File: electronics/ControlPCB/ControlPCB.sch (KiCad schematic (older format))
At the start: 29 parts, among them CON1 BARREL_JACK, P1 Opto1, P2 Opto2, P3 Opto3, P4 Opto4, P5 Opto5, P6 Opto6, P7 Tool, U1 POLOLU_A4988, U2 POLOLU_A4988, U3 POLOLU_A4988, U4 POLOLU_A4988, U5 POLOLU_A4988, U6 POLOLU_A4988, U7 POLOLU_A4988

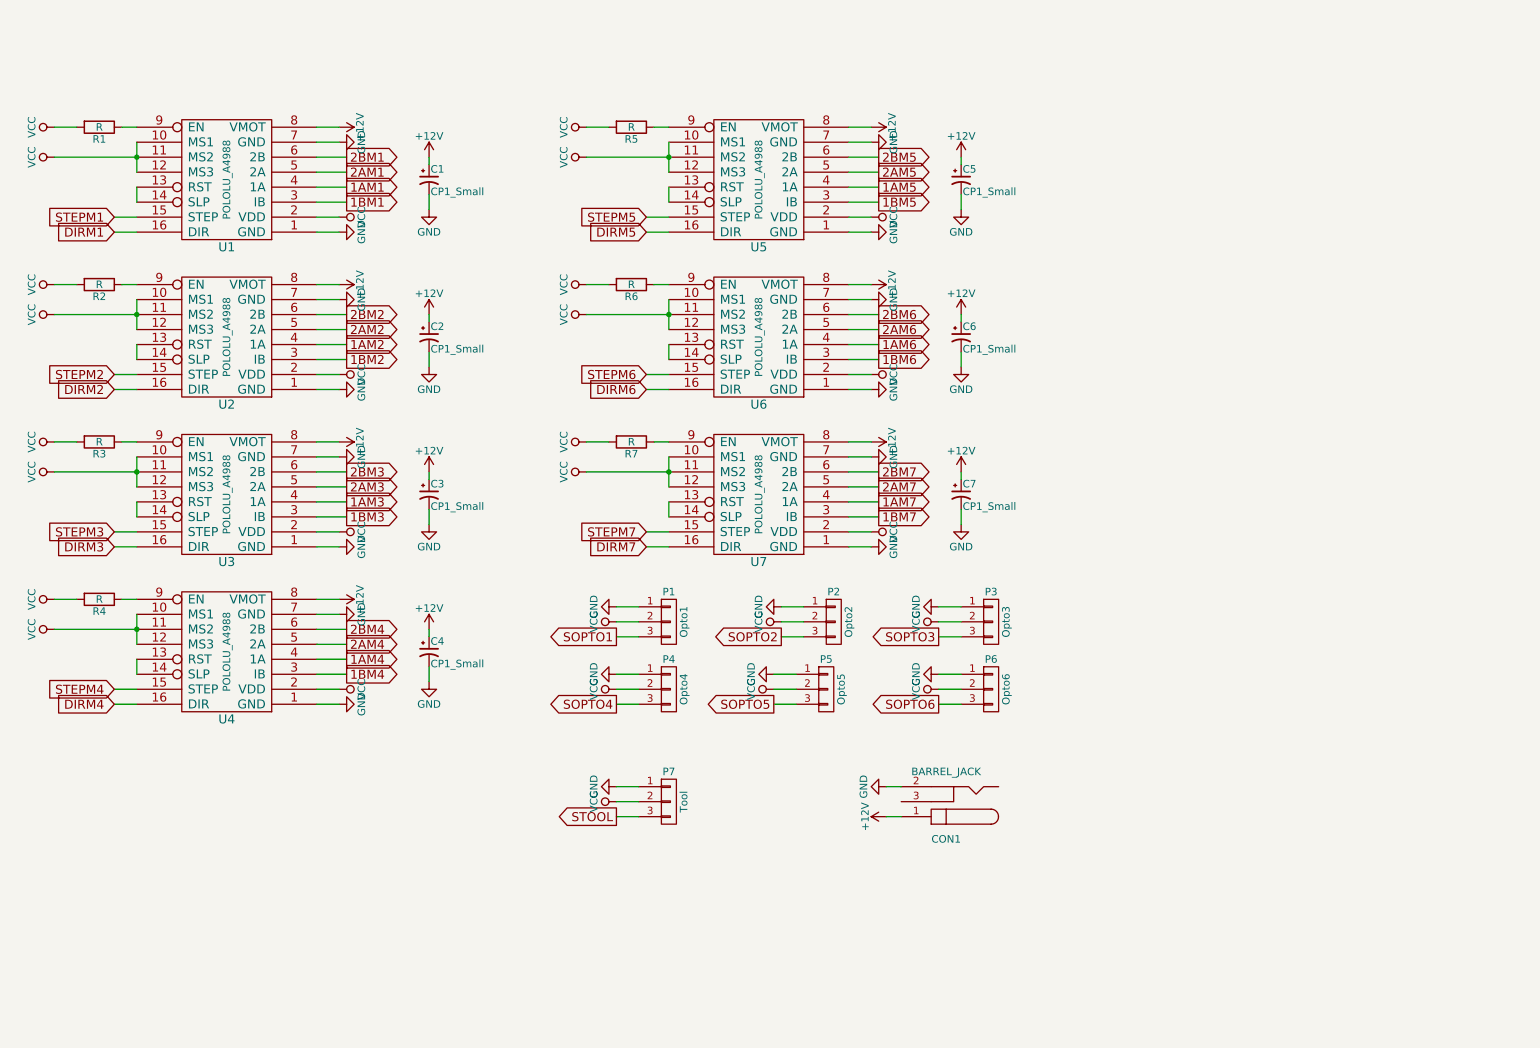
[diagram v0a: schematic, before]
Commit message: ControlPCB Kicad project update
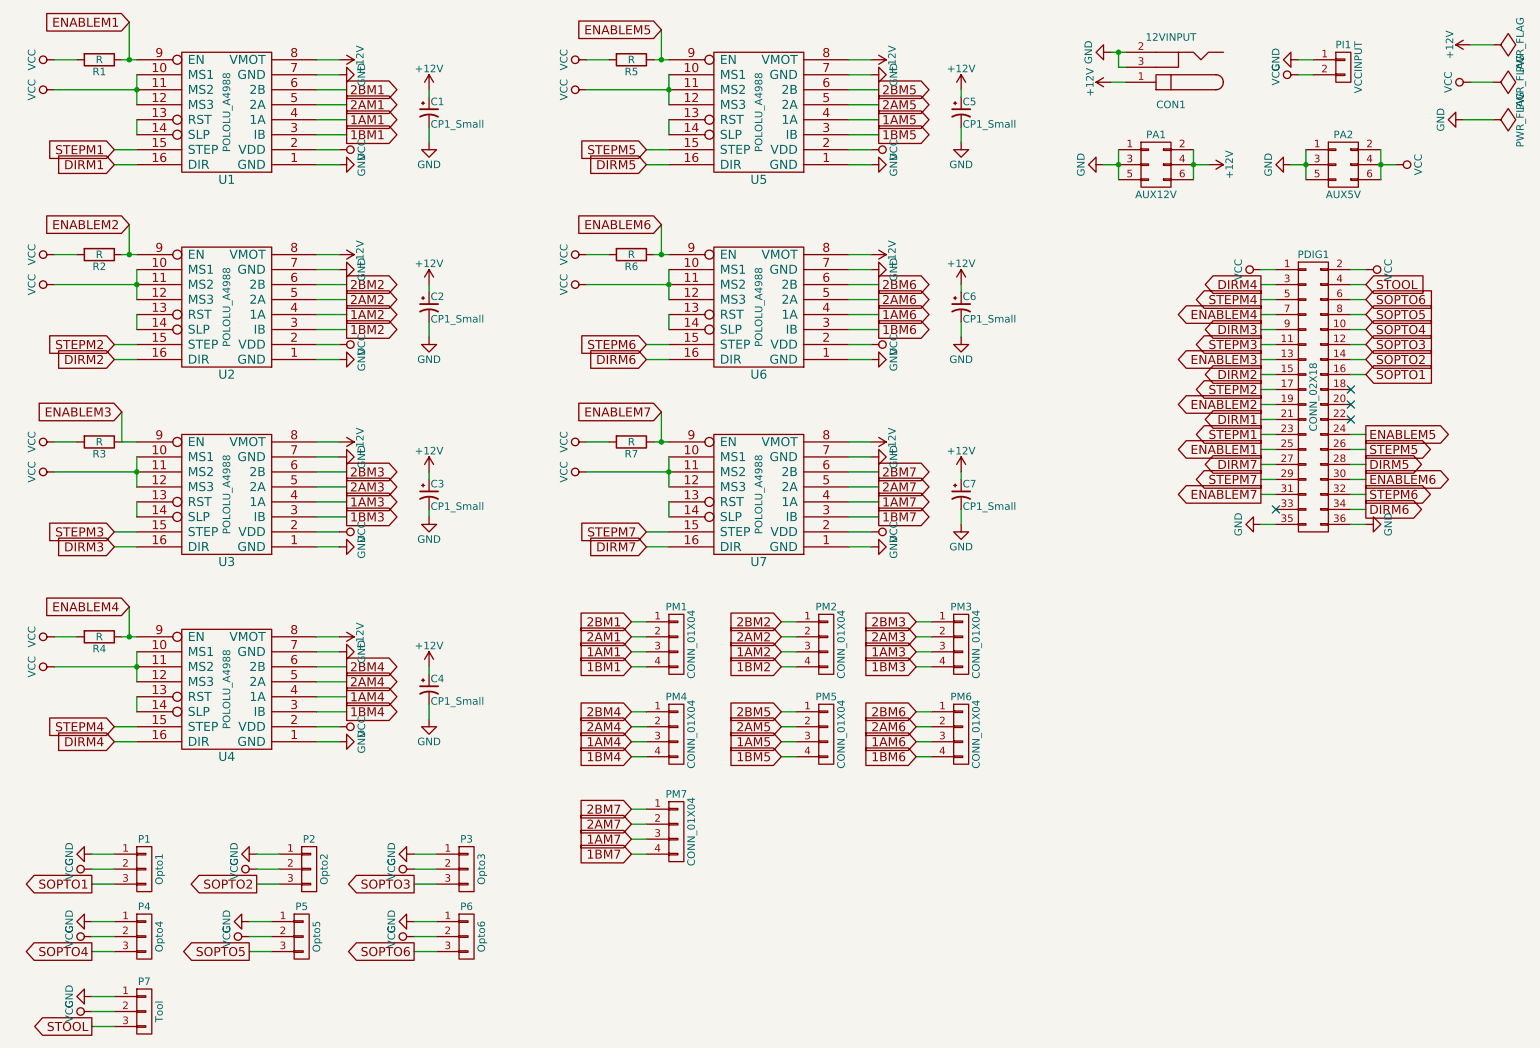
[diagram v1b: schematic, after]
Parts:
- added PA1: AUX12V, Pin_Headers:Pin_Header_Straight_2x03, symbol CONN_02X03
- added PA2: AUX5V, Pin_Headers:Pin_Header_Straight_2x03, symbol CONN_02X03
- added PDIG1: CONN_02X18, Pin_Headers:Pin_Header_Straight_2x18, symbol CONN_02X18
- added PI1: VCCINPUT, Pin_Headers:Pin_Header_Straight_1x02, symbol CONN_01X02
- added PM1, PM2, PM3, PM4, PM5, PM6, PM7: CONN_01X04, Pin_Headers:Pin_Header_Straight_1x04, symbol CONN_01X04
- C1, C2, C3, C4, C5, C6, C7: footprint (none) -> Capacitors_ThroughHole:C_Radial_D6.3_L11.2_P2.5
- CON1: value BARREL_JACK -> 12VINPUT; footprint (none) -> Connect:BARREL_JACK
- P1, P2, P3, P4, P5, P6, P7: footprint (none) -> Pin_Headers:Pin_Header_Straight_1x03
- R1, R2, R3, R4, R5, R6, R7: footprint (none) -> Resistors_ThroughHole:Resistor_Horizontal_RM7mm
- U1, U2, U3, U4, U5, U6, U7: footprint (none) -> POL:POLA4988
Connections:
- net +12V: now also PA1.2 (P2), PA1.4 (P4), PA1.6 (P6)
- net 1AM1: now also PM1.3 (P3)
- net 1AM2: now also PM2.3 (P3)
- net 1AM3: now also PM3.3 (P3)
- net 1AM4: now also PM4.3 (P3)
- net 1AM5: now also PM5.3 (P3)
- net 1AM6: now also PM6.3 (P3)
- net 1AM7: now also PM7.3 (P3)
- net 1BM1: now also PM1.4 (P4)
- net 1BM2: now also PM2.4 (P4)
- net 1BM3: now also PM3.4 (P4)
- net 1BM4: now also PM4.4 (P4)
- net 1BM5: now also PM5.4 (P4)
- net 1BM6: now also PM6.4 (P4)
- net 1BM7: now also PM7.4 (P4)
- net 2AM1: now also PM1.2 (P2)
- net 2AM2: now also PM2.2 (P2)
- net 2AM3: now also PM3.2 (P2)
- net 2AM4: now also PM4.2 (P2)
- net 2AM5: now also PM5.2 (P2)
- net 2AM6: now also PM6.2 (P2)
- net 2AM7: now also PM7.2 (P2)
- net 2BM1: now also PM1.1 (P1)
- net 2BM2: now also PM2.1 (P1)
- net 2BM3: now also PM3.1 (P1)
- net 2BM4: now also PM4.1 (P1)
- net 2BM5: now also PM5.1 (P1)
- net 2BM6: now also PM6.1 (P1)
- net 2BM7: now also PM7.1 (P1)
- net DIRM1: now also PDIG1.21 (P21)
- net DIRM2: now also PDIG1.15 (P15)
- net DIRM3: now also PDIG1.9 (P9)
- net DIRM4: now also PDIG1.3 (P3)
- net DIRM5: now also PDIG1.28 (P28)
- net DIRM6: now also PDIG1.34 (P34)
- net DIRM7: now also PDIG1.27 (P27)
- net GND: now also CON1.3, PA1.1 (P1), PA1.3 (P3), PA1.5 (P5), PA2.1 (P1), PA2.3 (P3), PA2.5 (P5), PDIG1.35 (P35), PDIG1.36 (P36), PI1.1 (P1)
- net SOPTO1: now also PDIG1.16 (P16)
- net SOPTO2: now also PDIG1.14 (P14)
- net SOPTO3: now also PDIG1.12 (P12)
- net SOPTO4: now also PDIG1.10 (P10)
- net SOPTO5: now also PDIG1.8 (P8)
- net SOPTO6: now also PDIG1.6 (P6)
- net STEPM1: now also PDIG1.23 (P23)
- net STEPM2: now also PDIG1.17 (P17)
- net STEPM3: now also PDIG1.11 (P11)
- net STEPM4: now also PDIG1.5 (P5)
- net STEPM5: now also PDIG1.26 (P26)
- net STEPM6: now also PDIG1.32 (P32)
- net STEPM7: now also PDIG1.29 (P29)
- net STOOL: now also PDIG1.4 (P4)
- net VCC: now also PA2.2 (P2), PA2.4 (P4), PA2.6 (P6), PDIG1.1 (P1), PDIG1.2 (P2), PI1.2 (P2)
- net ENABLEM1: now reaches R1.1, U1.9 (EN)
- net ENABLEM1: now also PDIG1.25 (P25)
- net ENABLEM2: now reaches R2.1, U2.9 (EN)
- net ENABLEM2: now also PDIG1.19 (P19)
- net ENABLEM3: now reaches R3.1, U3.9 (EN)
- net ENABLEM3: now also PDIG1.13 (P13)
- net ENABLEM4: now reaches R4.1, U4.9 (EN)
- net ENABLEM4: now also PDIG1.7 (P7)
- net ENABLEM5: now reaches R5.1, U5.9 (EN)
- net ENABLEM5: now also PDIG1.24 (P24)
- net ENABLEM6: now reaches R6.1, U6.9 (EN)
- net ENABLEM6: now also PDIG1.30 (P30)
- net ENABLEM7: now reaches R7.1, U7.9 (EN)
- net ENABLEM7: now also PDIG1.31 (P31)
- no-connect marks 0 -> 4
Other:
- moved on the sheet: C1, C2, C4, C5, C6, CON1, P1, P2, P3, P4, P5, P6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
